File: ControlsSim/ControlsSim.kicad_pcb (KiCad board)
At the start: 2 copper layers, 100 x 100 mm, 26 parts, among them J2 Accelerator Pot, J3 Brake Button, J5 Motor Contactors, J6 Array Contactors, J7 Rotary Switch, SW2 SW_Rotary2x6

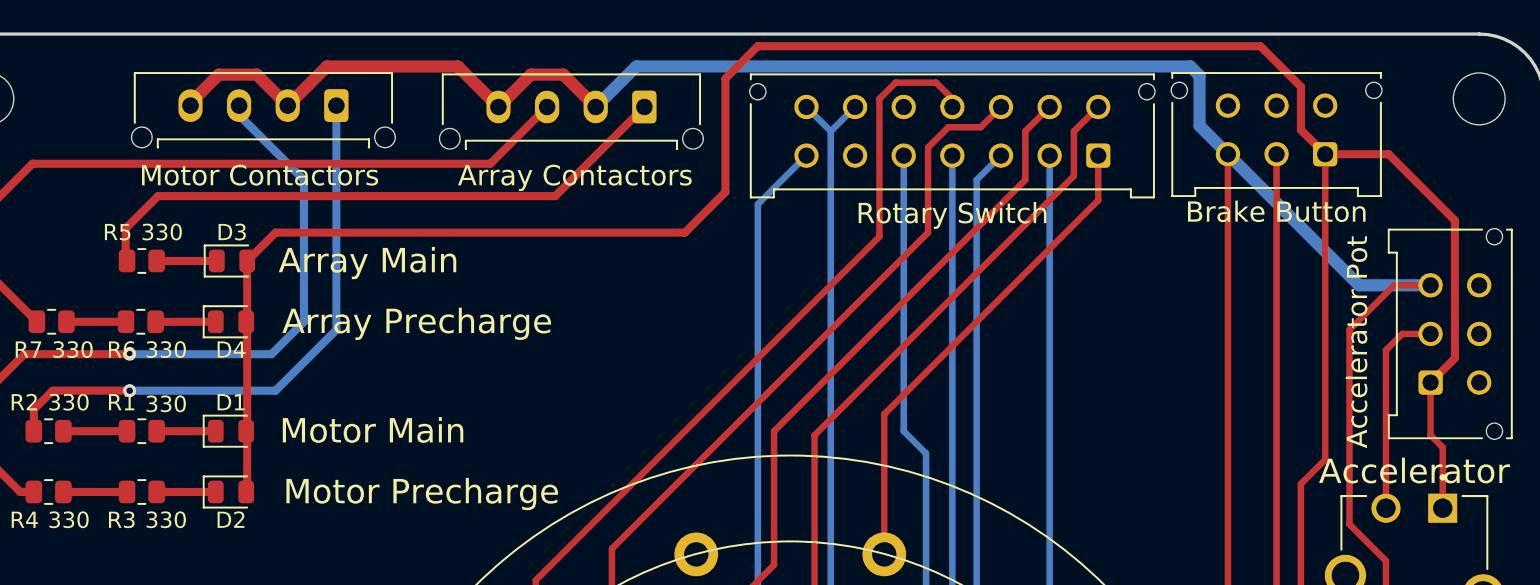
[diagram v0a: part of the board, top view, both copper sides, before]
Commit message: Beginning of Standardization
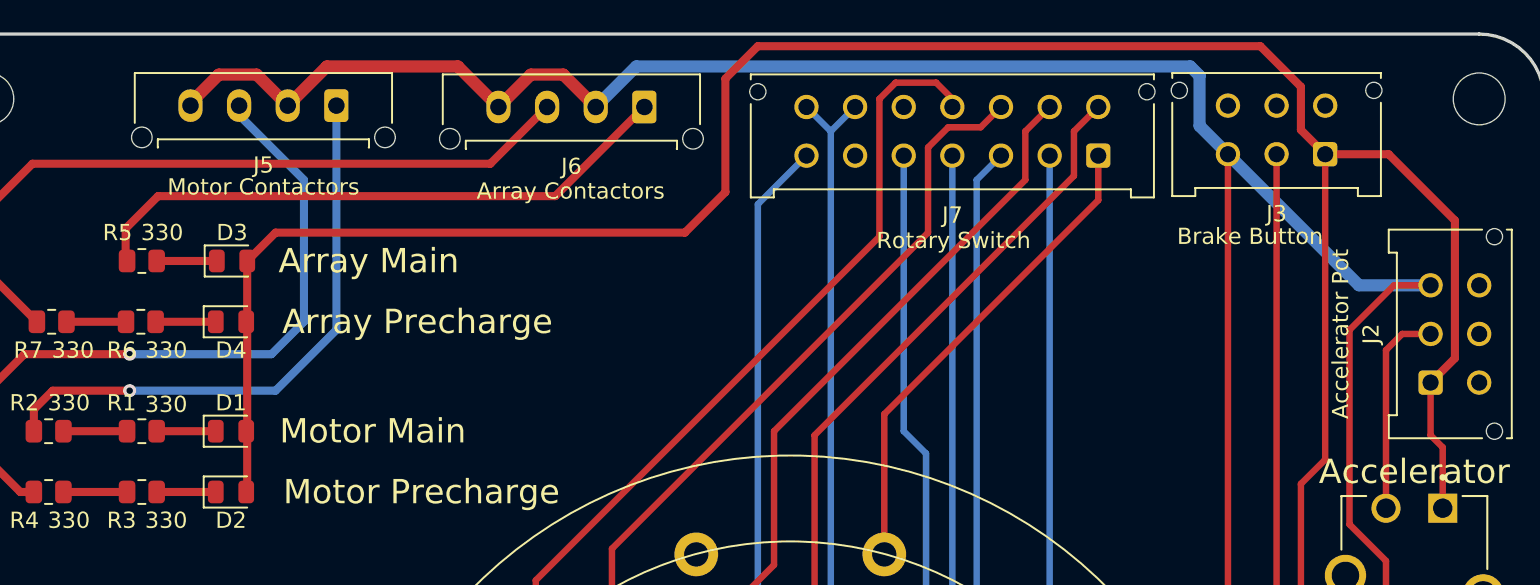
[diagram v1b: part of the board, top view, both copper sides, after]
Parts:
- J2, J3: footprint Connector_Molex:Molex_Micro-Fit_3.0_43045-0612_2x03_P3.00mm_Vertical -> UTSVT_Connectors:Molex_Micro-Fit_3.0_43045-0612_2x03_P3.00mm_Vertical
- J5, J6: footprint Connector_Molex:Molex_Micro-Fit_3.0_43650-0415_1x04_P3.00mm_Vertical -> UTSVT_Connectors:Molex_Micro-Fit_3.0_43650-0415_1x04_P3.00mm_Vertical
- J7: footprint Connector_Molex:Molex_Micro-Fit_3.0_43045-1412_2x07_P3.00mm_Vertical -> UTSVT_Connectors:Molex_Micro-Fit_3.0_43045-1412_2x07_P3.00mm_Vertical
